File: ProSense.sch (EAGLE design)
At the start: 24 parts, among them U4 MIC2505 3.3

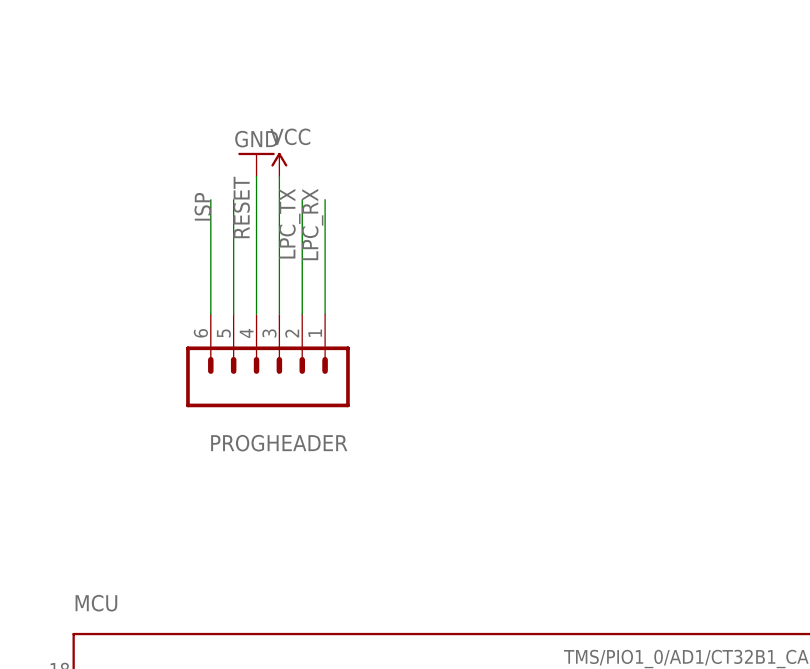
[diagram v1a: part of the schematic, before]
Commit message: fixup
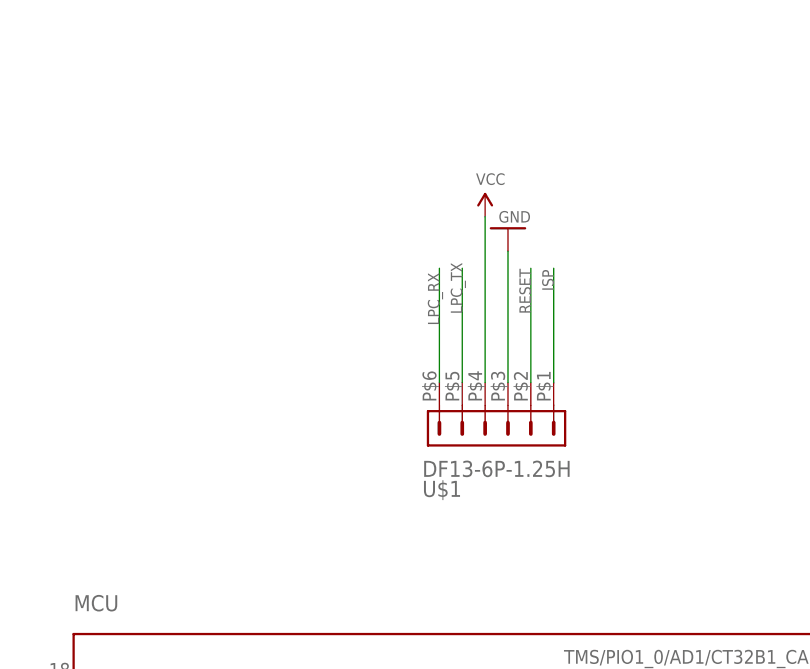
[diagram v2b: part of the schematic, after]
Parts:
- removed PROGHEADER: (no value), SparkFun-Connectors:M06LOCK
- added U$1: DF13-6P-1.25H, con-hirose-df13:DF13-6P-1.25H
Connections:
- net GND: now also U$1.3; no longer PROGHEADER.4
- net ISP: now also U$1.1; no longer PROGHEADER.6
- net LPC_RX: now also U$1.6; no longer PROGHEADER.1
- net LPC_TX: now also U$1.5; no longer PROGHEADER.2
- net RESET: now also U$1.2; no longer PROGHEADER.5
- net VCC: now also U$1.4; no longer PROGHEADER.3
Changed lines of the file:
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@@
 <setting verticaltext="up"/>
 </settings>
-<grid distance="0.1" unitdist="inch" unit="inch" style="lines" multiple="1" display="no" altdistance="0.01" altunitdist="inch" altunit="inch"/>
+<grid distance="0.025" unitdist="inch" unit="inch" style="lines" multiple="1" display="no" altdistance="0.01" altunitdist="inch" altunit="inch"/>
 <layers>
 <layer number="1" name="Top" color="4" fill="1" visible="no" active="no"/>
@@
 <part name="C5" library="SparkFun-Passives" deviceset="CAP" device="0805" value="4.7uF"/>
 <part name="GND5" library="SparkFun-Aesthetics" deviceset="GND" device=""/>
-<part name="SUPPLY14" library="SparkFun-Aesthetics" deviceset="VCC" device=""/>
-<part name="GND22" library="SparkFun-Aesthetics" deviceset="GND" device=""/>
 <part name="D1" library="SparkFun-LED" deviceset="LED-PURPLE" device="1206" value="PURPLE"/>
 <part name="R4" library="SparkFun-Passives" deviceset="RESISTOR" device="0805-RES" value="330"/>
@@
 <part name="SUPPLY1" library="SparkFun-Aesthetics" deviceset="V_BATT" device=""/>
 <part name="SUPPLY18" library="SparkFun-Aesthetics" deviceset="VCC" device=""/>
-<part name="PROGHEADER" library="SparkFun-Connectors" deviceset="M06" device="LOCK"/>
 <part name="MCU" library="NXP_60_26022015" deviceset="LPC1112FD20" device="" technology="/102"/>
+<part name="U$1" library="con-hirose-df13" deviceset="DF13-6P-1.25" device="H"/>
+<part name="GND7" library="SparkFun-Aesthetics" deviceset="GND" device=""/>
+<part name="SUPPLY13" library="SparkFun-Aesthetics" deviceset="VCC" device=""/>
 </parts>
 <sheets>
@@
 </instance>
 <instance part="GND5" gate="1" x="21.59" y="57.15" rot="R180"/>
-<instance part="SUPPLY14" gate="G$1" x="0" y="180.34"/>
-<instance part="GND22" gate="1" x="-2.54" y="182.88" rot="R180"/>
 <instance part="D1" gate="G$1" x="-147.32" y="76.2" smashed="yes" rot="R270">
 <attribute name="NAME" x="-155.702" y="73.914" size="1.778" layer="95"/>
@@
 <instance part="SUPPLY1" gate="G$1" x="154.94" y="81.28"/>
 <instance part="SUPPLY18" gate="G$1" x="-132.08" y="106.68" rot="MR270"/>
-<instance part="PROGHEADER" gate="G$1" x="0" y="160.02" smashed="yes" rot="R90">
-<attribute name="VALUE" x="10.16" y="154.94" size="1.778" layer="96" rot="R90"/>
-<attribute name="NAME" x="7.62" y="151.638" size="1.778" layer="95" rot="R180"/>
-</instance>
 <instance part="MCU" gate="G$1" x="20.32" y="106.68"/>
+<instance part="U$1" gate="G$1" x="25.4" y="152.4" smashed="yes" rot="R270">
+<attribute name="NAME" x="15.875" y="144.78" size="1.778" layer="95"/>
+<attribute name="VALUE" x="15.875" y="147.0025" size="1.778" layer="96"/>
+</instance>
+<instance part="GND7" gate="1" x="25.4" y="174.625" smashed="yes" rot="R180">
+<attribute name="VALUE" x="27.94" y="176.53" size="1.27" layer="96" rot="R180"/>
+</instance>
+<instance part="SUPPLY13" gate="G$1" x="22.86" y="175.895" smashed="yes">
+<attribute name="VALUE" x="21.844" y="179.451" size="1.27" layer="96"/>
+</instance>
 </instances>
 <busses>
@@
 <pinref part="SUPPLY12" gate="G$1" pin="VCC"/>
 <wire x1="-21.59" y1="16.51" x2="-8.89" y2="16.51" width="0.1524" layer="91"/>
-</segment>
-<segment>
-<pinref part="SUPPLY14" gate="G$1" pin="VCC"/>
-<wire x1="0" y1="180.34" x2="0" y2="165.1" width="0.1524" layer="91"/>
-<pinref part="PROGHEADER" gate="G$1" pin="3"/>
 </segment>
 <segment>
@@
 <pinref part="C8" gate="G$1" pin="1"/>
 <junction x="-38.1" y="96.52"/>
+</segment>
+<segment>
+<pinref part="U$1" gate="G$1" pin="4"/>
+<wire x1="22.86" y1="157.48" x2="22.86" y2="175.895" width="0.1524" layer="91"/>
+<pinref part="SUPPLY13" gate="G$1" pin="VCC"/>
 </segment>
 </net>
@@
 </segment>
 <segment>
-<pinref part="GND22" gate="1" pin="GND"/>
-<wire x1="-2.54" y1="180.34" x2="-2.54" y2="165.1" width="0.1524" layer="91"/>
-<pinref part="PROGHEADER" gate="G$1" pin="4"/>
-</segment>
-<segment>
 <pinref part="BNO180" gate="G$1" pin="GND"/>
 <wire x1="-46.99" y1="19.05" x2="-44.45" y2="19.05" width="0.1524" layer="91"/>
@@
 <wire x1="-38.1" y1="88.9" x2="-38.1" y2="83.82" width="0.1524" layer="91"/>
 <junction x="-38.1" y="88.9"/>
+</segment>
+<segment>
+<pinref part="U$1" gate="G$1" pin="3"/>
+<wire x1="25.4" y1="157.48" x2="25.4" y2="172.085" width="0.1524" layer="91"/>
+<pinref part="GND7" gate="1" pin="GND"/>
 </segment>
 </net>
@@
 </segment>
 <segment>
-<label x="2.54" y="179.07" size="1.778" layer="95" rot="R270"/>
-<wire x1="5.08" y1="165.1" x2="5.08" y2="177.8" width="0.1524" layer="91"/>
-<pinref part="PROGHEADER" gate="G$1" pin="1"/>
+<wire x1="17.78" y1="157.48" x2="17.78" y2="170.18" width="0.1524" layer="91"/>
+<label x="17.78" y="163.83" size="1.27" layer="95" rot="R90"/>
+<pinref part="U$1" gate="G$1" pin="6"/>
 </segment>
 <segment>
@@
 </segment>
 <segment>
-<label x="0" y="179.07" size="1.778" layer="95" rot="R270"/>
-<wire x1="2.54" y1="165.1" x2="2.54" y2="177.8" width="0.1524" layer="91"/>
-<pinref part="PROGHEADER" gate="G$1" pin="2"/>
+<label x="19.05" y="170.815" size="1.27" layer="95" rot="R270"/>
+<wire x1="20.32" y1="157.48" x2="20.32" y2="170.18" width="0.1524" layer="91"/>
+<pinref part="U$1" gate="G$1" pin="5"/>
 </segment>
 <segment>
@@
 </segment>
 <segment>
-<pinref part="PROGHEADER" gate="G$1" pin="6"/>
-<wire x1="-7.62" y1="165.1" x2="-7.62" y2="177.8" width="0.1524" layer="91"/>
-<label x="-7.62" y="175.26" size="1.778" layer="95" rot="R90"/>
+<wire x1="30.48" y1="157.48" x2="30.48" y2="170.18" width="0.1524" layer="91"/>
+<label x="30.48" y="167.64" size="1.27" layer="95" rot="R90"/>
+<pinref part="U$1" gate="G$1" pin="1"/>
 </segment>
 </net>
@@
 </segment>
 <segment>
-<pinref part="PROGHEADER" gate="G$1" pin="5"/>
-<wire x1="-5.08" y1="165.1" x2="-5.08" y2="177.8" width="0.1524" layer="91"/>
-<label x="-5.08" y="180.34" size="1.778" layer="95" rot="R270"/>
-</segment>
-</net>
+<wire x1="27.94" y1="157.48" x2="27.94" y2="170.18" width="0.1524" layer="91"/>
+<pinref part="U$1" gate="G$1" pin="2"/>
+<label x="27.94" y="165.1" size="1.27" layer="95" rot="R90"/>
+</segment>
+</net>

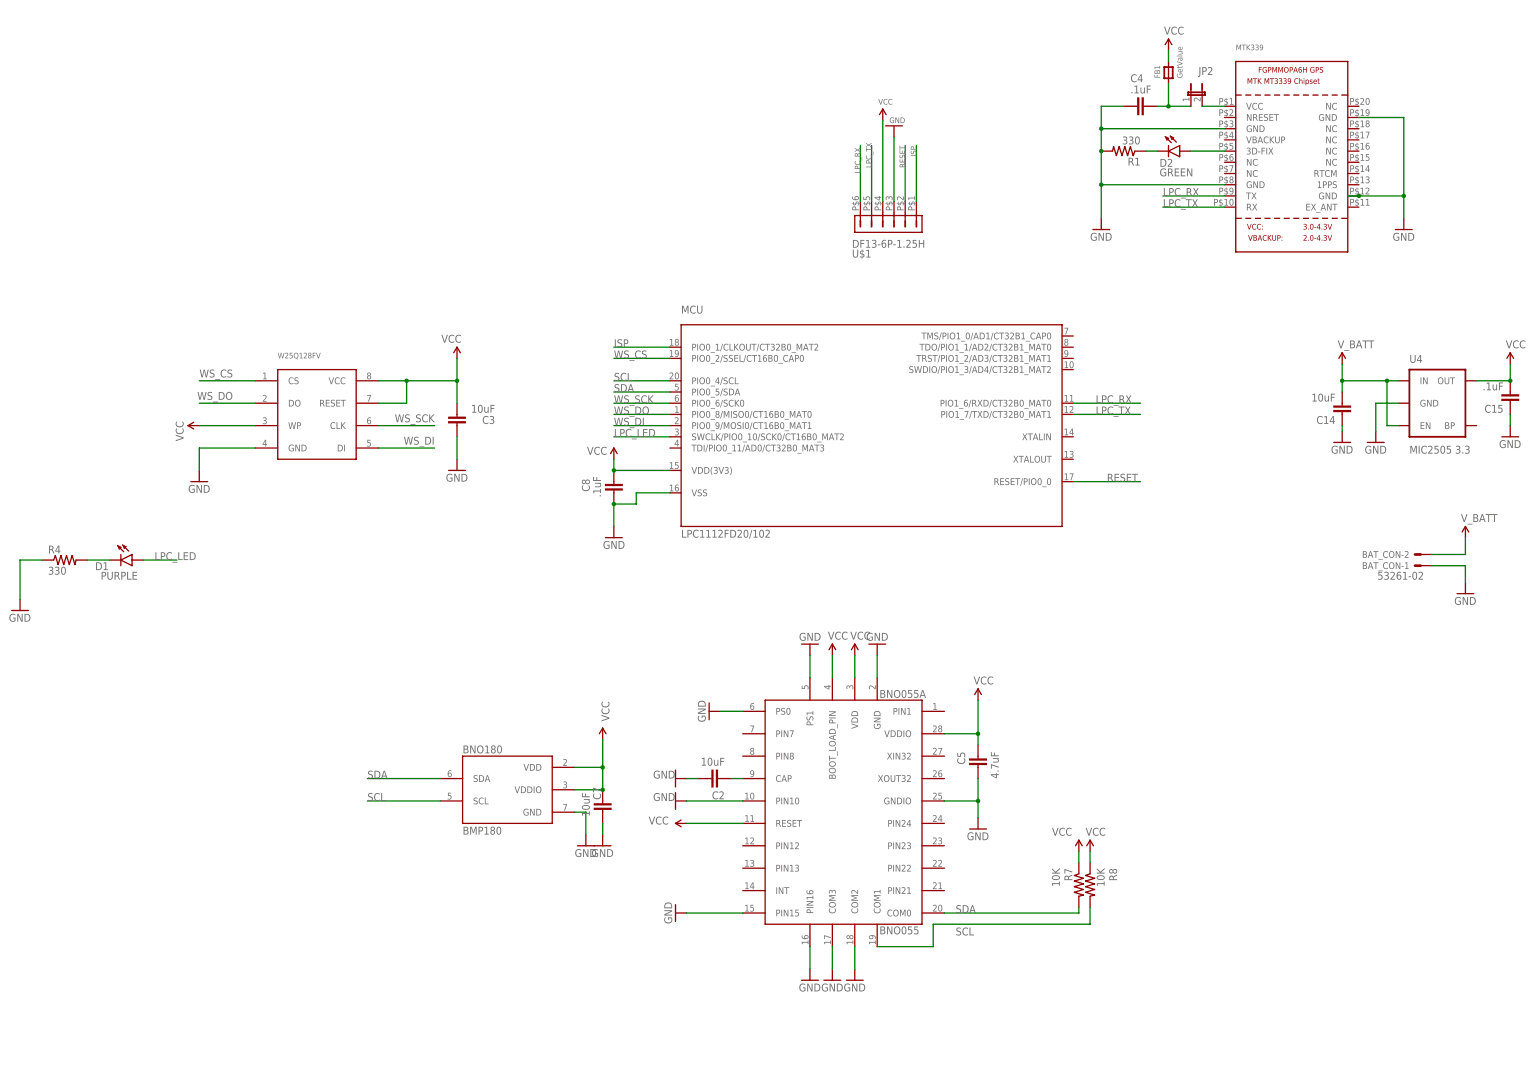
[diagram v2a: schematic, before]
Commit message: Finished rev 1.2.1
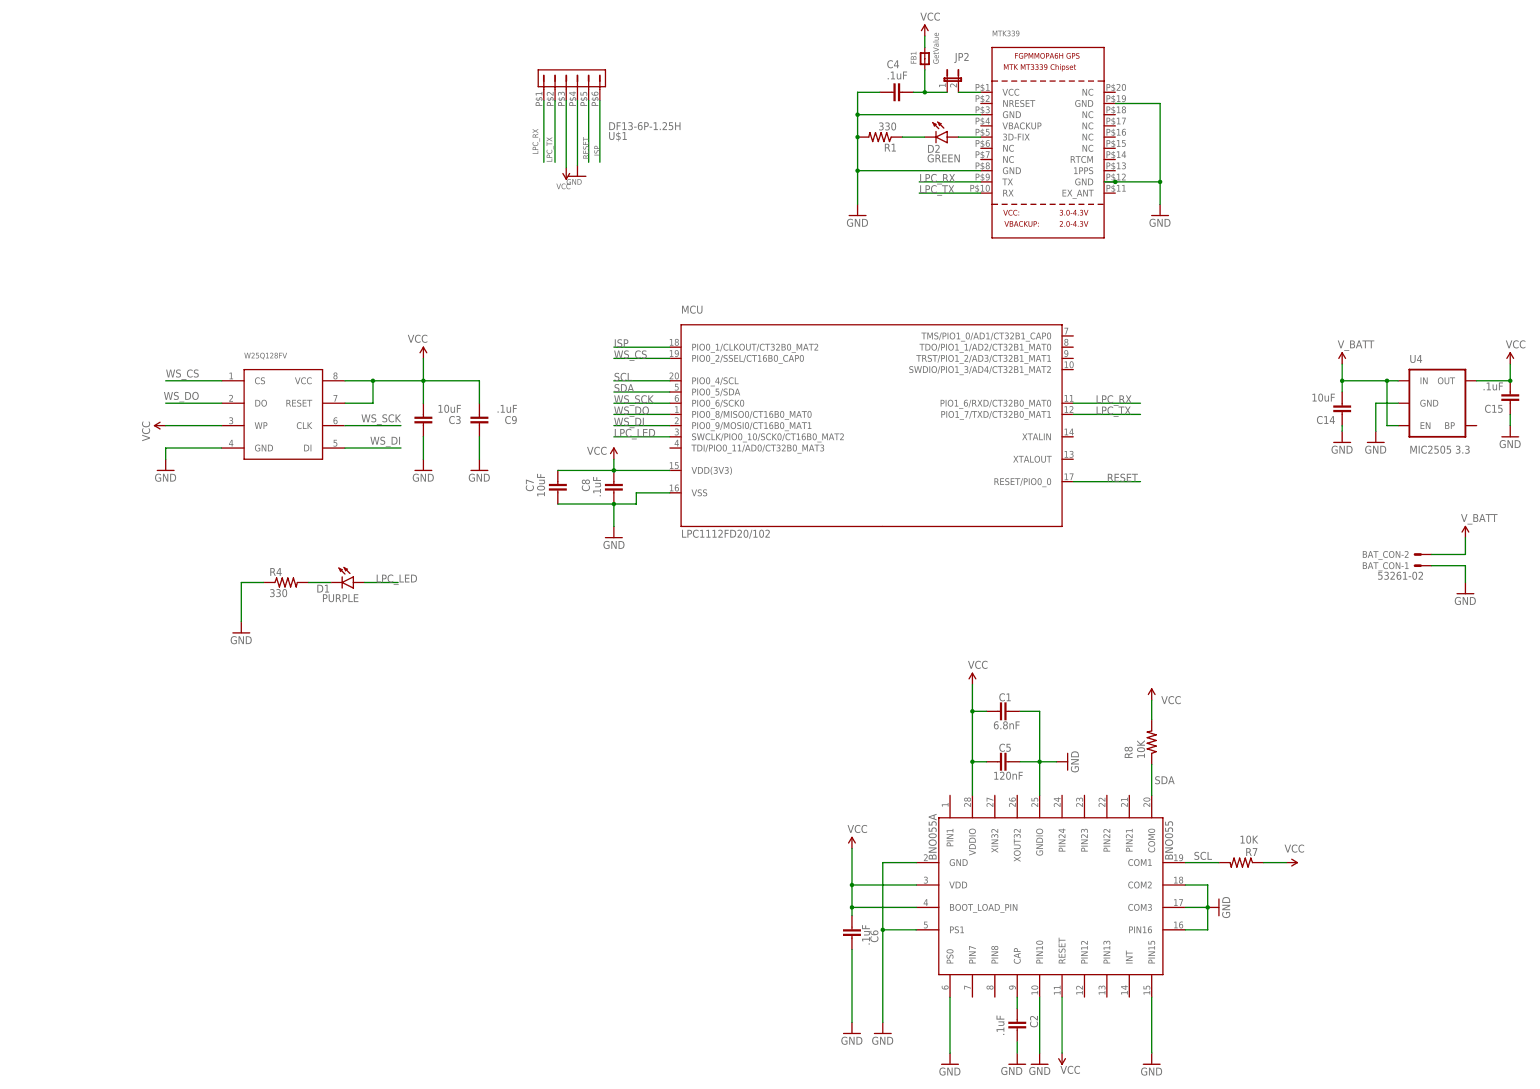
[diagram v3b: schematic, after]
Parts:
- removed BNO180: BMP180, SparkFun-Sensors:BMP180
- added C1: 6.8nF, SparkFun-Passives:CAP0805
- added C6, C9: .1uF, SparkFun-Passives:CAP0805
- C2: value 10uF -> .1uF
- C5: value 4.7uF -> 120nF
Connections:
- net N$6 renamed GPS-LED
- net GND: now also C1.1, C6.2, C9.1, U$1.4; no longer BNO180.GND, U$1.3
- net ISP: now also U$1.6; no longer U$1.1
- net LPC_RX: now also U$1.1; no longer U$1.6
- net LPC_TX: now also U$1.2; no longer U$1.5
- net RESET: now also U$1.5; no longer U$1.2
- net SCL: now also R7.2; no longer BNO180.SCL, R8.2
- net SDA: now also R8.1; no longer BNO180.SDA, R7.2
- net VCC: now also C1.2, C6.1, C9.2, R8.2, U$1.3; no longer BNO180.VDD, BNO180.VDDIO, R8.1, U$1.4
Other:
- moved on the sheet: BNO055, C2, C3, C4, C5, C7, D1, D2, FB1, JP2, MTK339, R1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
